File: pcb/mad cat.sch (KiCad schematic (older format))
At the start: 274 parts, among them J1 Conn_01x04, J2 Conn_02x03_Odd_Even, SW0,0 ESC, SW0,1 ESC/F1, SW0,10 F9, SW0,10-1 F10, SW0,11 F10, SW0,11-1 F11, SW0,12 F11, SW0,12-1 F12, SW0,13 F12/PRT, SW0,14 INS, SW0,15 HOME, SW0,16 PGUP, SW0,2 F1, SW0,2-1 F2, SW0,3 F2, SW0,3-1 F3, SW0,4 F3, SW0,4-1 F4, SW0,5 F4, SW0,5-1 F5, SW0,6 F5, SW0,6-1 F6, SW0,7 F6, SW0,7-1 F7, SW0,8 F7, SW0,8-1 F8, SW0,9 F8, SW0,9-1 F9, SW1,0 PF1, SW1,0-1 PF1, SW1,1 TILDE, SW1,10 9, SW1,11 0, SW1,12 -, SW1,13 =, SW1,14 BACKSPACE, SW1,14-1 S_BS_L, SW1,15 END, SW1,16 PGDN, SW1,2 1, SW1,3 2, SW1,4 3, SW1,5 4, SW1,6 5, SW1,7 6, SW1,8 7, SW1,9 8, SW2,0 PF2, SW2,0-1 PF2, SW2,1 TAB, SW2,10 O, SW2,11 P, SW2,12 [, SW2,13 ], SW2,14 \\, SW2,15 S_BS_R, SW2,16 PRT, SW2,2 Q, SW2,3 W, SW2,4 E, SW2,5 R, SW2,6 T, SW2,7 Y, SW2,8 U, SW2,9 I, SW3,0 PF3, SW3,0-1 PF3, SW3,1 CAPS, SW3,1-1 ST_CAPS, SW3,10 L, SW3,11 COLONS, SW3,12 QUOTE, SW3,13 ISO_#, SW3,14 ENT, SW3,14-1 ISO_ENT, SW3,15 DEL, SW3,15-1 DEL, SW3,15-2 DEL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

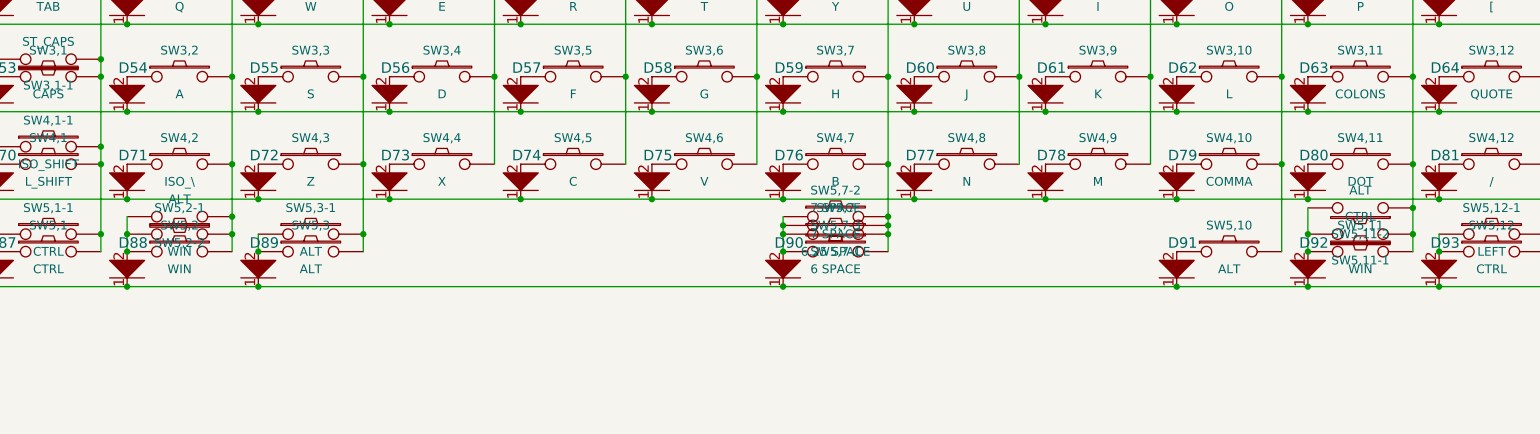
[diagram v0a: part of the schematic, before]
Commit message: design done for proto
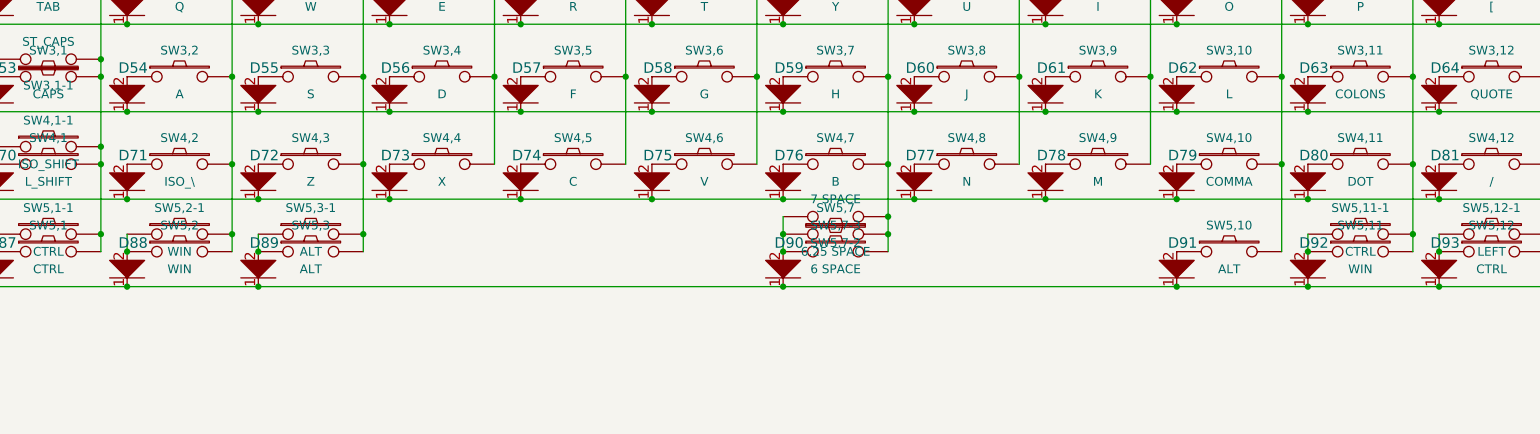
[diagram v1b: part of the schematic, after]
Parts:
- removed SW5,11-2, SW5,2-2: ALT, MX_SMK_2:MX_150, symbol keyboard_parts:SW_PUSH
- removed SW5,7-1: 7 SPACE, MX_SMK_2:MX_700_stabflip, symbol keyboard_parts:SW_PUSH
- EC1, EC2: footprint keebs:EC11E -> keebs:EC11E_offset
- SW5,7-2: footprint MX_SMK_2:MX_700_stabflip -> MX_SMK_2:MX_100
- SW5,7-3: footprint MX_SMK_2:MX_100 -> MX_SMK_2:MX_600_stabflip
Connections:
- net c11: now also SW5,11-1.2; no longer SW5,11-1.1
- net c7: now also SW5,7-2.1; no longer SW5,7-2.2
- net at D90.2, SW5,7-3.1, SW5,7.1: now also SW5,7-2.2; no longer SW5,7-2.1
- net at D92.2, SW5,11.1: now also SW5,11-1.1; no longer SW5,11-1.2
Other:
- moved on the sheet: SW5,11-1, SW5,7-2
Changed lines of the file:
@@
 F 0 "EC2" H 13800 2083 50  0000 C CNN
 F 1 "EC11E" H 13800 2174 50  0000 C CNN
-F 2 "keebs:EC11E" H 13650 2610 50  0001 C CNN
+F 2 "keebs:EC11E_offset" H 13650 2610 50  0001 C CNN
 F 3 "~" H 13800 2710 50  0001 C CNN
 	1    13800 2450
@@
 F 0 "EC1" V 804 1180 50  0000 L CNN
 F 1 "EC11E" V 895 1180 50  0000 L CNN
-F 2 "keebs:EC11E" H 700 1110 50  0001 C CNN
+F 2 "keebs:EC11E_offset" H 700 1110 50  0001 C CNN
 F 3 "~" H 850 1210 50  0001 C CNN
 	1    850  950
@@
 	-1   0    0    1
 $EndComp
-Wire Wire Line
-	6600 4050 6600 3950
 Connection ~ 6600 1550
 Connection ~ 6600 2050
@@
 	-1   0    0    1
 $EndComp
-Wire Wire Line
-	9600 4050 9600 3950
 Connection ~ 9600 1550
 Wire Wire Line
@@
 	1    0    0    -1
 $EndComp
-Connection ~ 6600 3950
-Wire Wire Line
-	6600 3950 6600 3900
 Wire Wire Line
 	6000 3950 6000 4050
@@
 F 3 "" H 9300 3950 60  0000 C CNN
 	1    9300 3950
-	-1   0    0    1
+	1    0    0    -1
 $EndComp
 $Comp
@@
 Connection ~ 2850 3950
 Wire Wire Line
-	2850 3950 2850 3850
-Wire Wire Line
 	2250 3950 2250 4050
 Connection ~ 2250 4050
@@
 Connection ~ 12000 3050
 $Comp
-L keyboard_parts:SW_PUSH SW5,11-2
-U 1 1 5CE261EE
-P 9300 3800
-F 0 "SW5,11-2" H 9300 3950 50  0000 C CNN
-F 1 "ALT" H 9300 3700 50  0000 C CNN
-F 2 "MX_SMK_2:MX_150" H 9300 3800 60  0001 C CNN
-F 3 "" H 9300 3800 60  0000 C CNN
-	1    9300 3800
-	-1   0    0    1
-$EndComp
-$Comp
 L keyboard_parts:SW_PUSH SW5,7-2
 U 1 1 5CE4437C
@@
 F 0 "SW5,7-2" H 6300 4000 50  0000 C CNN
 F 1 "7 SPACE" H 6300 3750 50  0000 C CNN
-F 2 "MX_SMK_2:MX_700_stabflip" H 6300 3850 60  0001 C CNN
+F 2 "MX_SMK_2:MX_100" H 6300 3850 60  0001 C CNN
 F 3 "" H 6300 3850 60  0000 C CNN
 	1    6300 3850
-	1    0    0    -1
-$EndComp
-Connection ~ 6600 3850
-Wire Wire Line
-	6600 3850 6600 3550
-Wire Wire Line
-	6000 3850 6000 3900
-Connection ~ 6000 3950
-$Comp
-L keyboard_parts:SW_PUSH SW5,2-2
-U 1 1 5CDD1EA0
-P 2550 3850
-F 0 "SW5,2-2" H 2550 4000 50  0000 C CNN
-F 1 "ALT" H 2550 3750 50  0000 C CNN
-F 2 "MX_SMK_2:MX_150" H 2550 3850 60  0001 C CNN
-F 3 "" H 2550 3850 60  0000 C CNN
-	1    2550 3850
-	-1   0    0    1
-$EndComp
-Connection ~ 2850 3850
-Wire Wire Line
-	2850 3850 2850 3550
-Wire Wire Line
-	2250 3850 2250 3950
-Connection ~ 2250 3950
-$Comp
-L keyboard_parts:SW_PUSH SW5,7-1
-U 1 1 5CDF148D
-P 6300 3900
-F 0 "SW5,7-1" H 6300 4050 50  0000 C CNN
-F 1 "7 SPACE" H 6300 3800 50  0000 C CNN
-F 2 "MX_SMK_2:MX_700_stabflip" H 6300 3900 60  0001 C CNN
-F 3 "" H 6300 3900 60  0000 C CNN
-	1    6300 3900
 	-1   0    0    1
 $EndComp
-Connection ~ 6600 3900
-Wire Wire Line
-	6600 3900 6600 3850
-Connection ~ 6000 3900
-Wire Wire Line
-	6000 3900 6000 3950
+Connection ~ 6000 3950
 $Comp
 L mad-cat-rescue:TC33X-2-103E-dk_Trimmer-Potentiometers POT1
@@
 Connection ~ 8850 3550
 Connection ~ 9000 4250
-Connection ~ 9600 3800
-Wire Wire Line
-	9600 3800 9600 3550
-Connection ~ 9600 3950
-Wire Wire Line
-	9600 3950 9600 3800
-Wire Wire Line
-	9000 4250 9750 4250
-Wire Wire Line
-	9000 3800 9000 3950
 Wire Wire Line
 	10350 3550 10350 3950
-Connection ~ 9000 3950
 Wire Wire Line
 	9000 3950 9000 4050
@@
 	1    0    0    -1
 $EndComp
+Wire Wire Line
+	11250 4250 12000 4250
+Connection ~ 12000 4250
+Wire Wire Line
+	12000 4250 12750 4250
 $Comp
 L keyboard_parts:SW_PUSH SW5,7-3
-U 1 1 5D89B8C2
+U 1 1 5D08BA56
 P 6300 4050
 F 0 "SW5,7-3" H 6300 4200 50  0000 C CNN
 F 1 "6 SPACE" H 6300 3950 50  0000 C CNN
-F 2 "MX_SMK_2:MX_100" H 6300 3950 60  0001 C CNN
+F 2 "MX_SMK_2:MX_600_stabflip" H 6300 4050 60  0001 C CNN
 F 3 "" H 6300 4050 60  0000 C CNN
 	1    6300 4050
@@
 Connection ~ 6000 4050
 Wire Wire Line
-	11250 4250 12000 4250
-Connection ~ 12000 4250
+	6600 3950 6600 4050
+Connection ~ 6600 3950
 Wire Wire Line
-	12000 4250 12750 4250
+	2850 3550 2850 3950
+Wire Wire Line
+	6000 3850 6000 3950
+Wire Wire Line
+	6600 3550 6600 3850
+Connection ~ 6600 3850
+Wire Wire Line
+	6600 3850 6600 3950
+Wire Wire Line
+	9600 3550 9600 3950
+Connection ~ 9600 3950
+Wire Wire Line
+	9600 3950 9600 4050
+Wire Wire Line
+	9000 4250 9750 4250
 $EndSCHEMATC

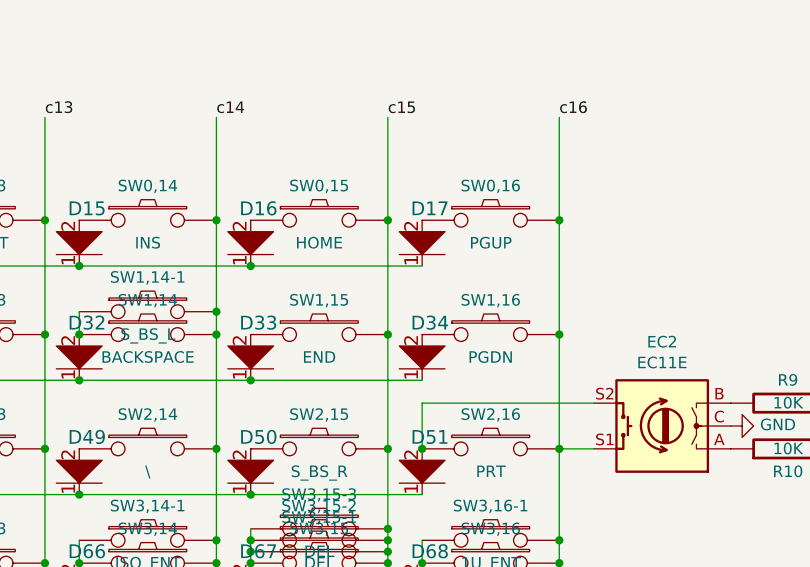
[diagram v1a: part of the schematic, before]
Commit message: back to editing pcb
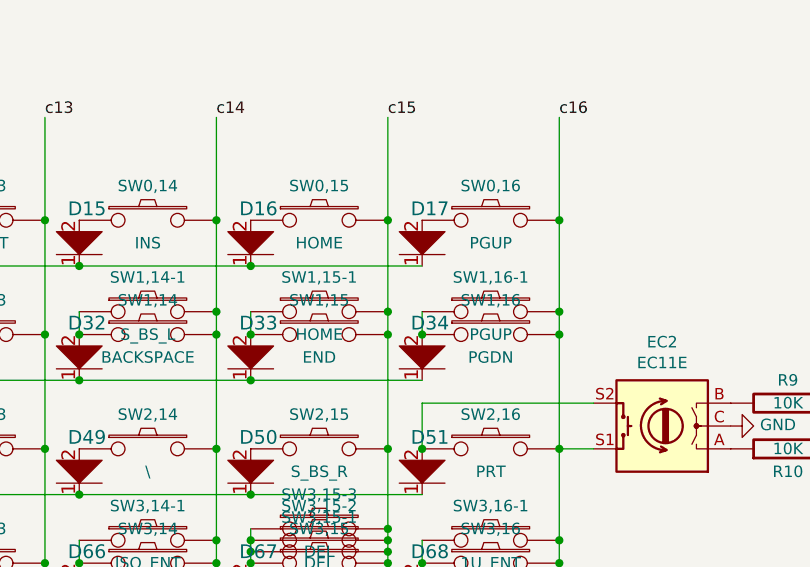
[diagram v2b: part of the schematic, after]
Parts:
- added SW1,15-1: HOME, MX_SMK_2:MX_100, symbol keyboard_parts:SW_PUSH
- added SW1,16-1: PGUP, MX_SMK_2:MX_100, symbol keyboard_parts:SW_PUSH
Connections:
- net c15: now also SW1,15-1.2
- net c16: now also SW1,16-1.2
- net at D33.2, SW1,15.1: now also SW1,15-1.1
- net at D34.2, SW1,16.1: now also SW1,16-1.1
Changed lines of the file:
@@
 Connection ~ 12600 2050
 Wire Wire Line
-	12600 2050 12600 1550
+	12600 2050 12600 1950
 Connection ~ 12600 2550
 Wire Wire Line
@@
 Connection ~ 13350 2050
 Wire Wire Line
-	13350 2050 13350 1550
+	13350 2050 13350 1950
 Connection ~ 13350 2550
 Connection ~ 13350 3050
@@
 Wire Wire Line
 	9000 4250 9750 4250
+$Comp
+L keyboard_parts:SW_PUSH SW1,16-1
+U 1 1 5D092AB2
+P 13050 1950
+F 0 "SW1,16-1" H 13050 2100 50  0000 C CNN
+F 1 "PGUP" H 13050 1850 50  0000 C CNN
+F 2 "MX_SMK_2:MX_100" H 13050 1950 60  0001 C CNN
+F 3 "" H 13050 1950 60  0000 C CNN
+	1    13050 1950
+	1    0    0    -1
+$EndComp
+Connection ~ 13350 1950
+Wire Wire Line
+	13350 1950 13350 1550
+Wire Wire Line
+	12750 1950 12750 2050
+Connection ~ 12750 2050
+$Comp
+L keyboard_parts:SW_PUSH SW1,15-1
+U 1 1 5D0B2107
+P 12300 1950
+F 0 "SW1,15-1" H 12300 2100 50  0000 C CNN
+F 1 "HOME" H 12300 1850 50  0000 C CNN
+F 2 "MX_SMK_2:MX_100" H 12300 1950 60  0001 C CNN
+F 3 "" H 12300 1950 60  0000 C CNN
+	1    12300 1950
+	1    0    0    -1
+$EndComp
+Connection ~ 12600 1950
+Wire Wire Line
+	12600 1950 12600 1550
+Wire Wire Line
+	12000 1950 12000 2050
+Connection ~ 12000 2050
 $EndSCHEMATC
